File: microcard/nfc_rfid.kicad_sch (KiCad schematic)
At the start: 39 parts, among them Q7 2N7002, U6 ST25R3916-AQWT, X1 XRCGB27M120F3M00R0

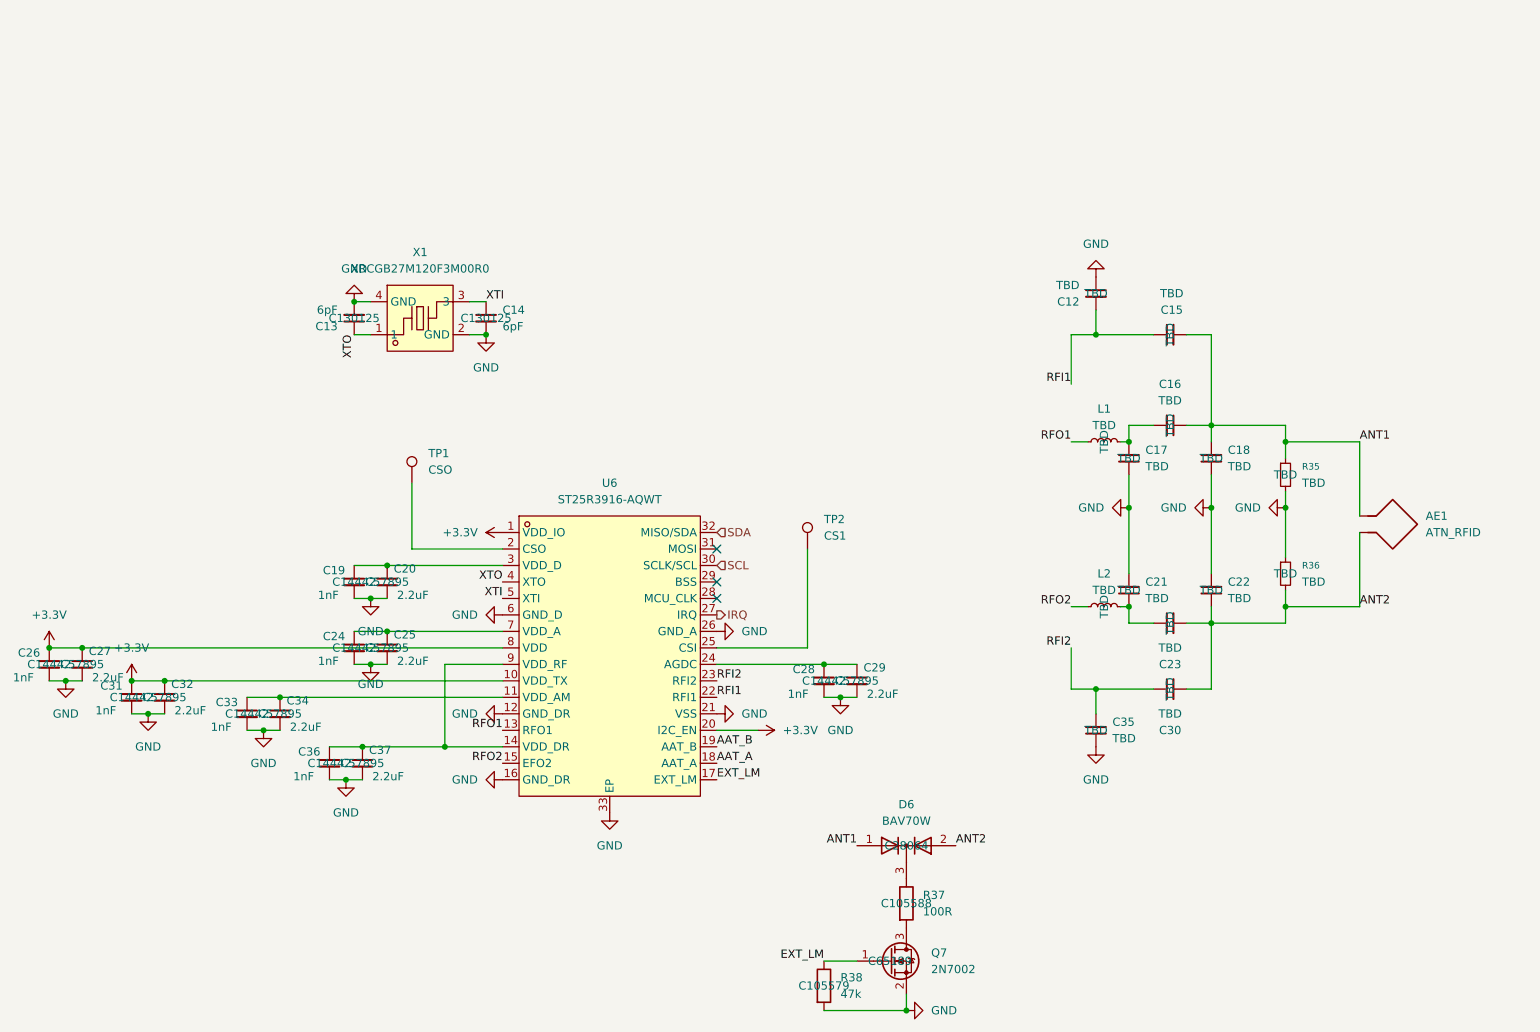
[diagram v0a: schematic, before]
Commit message: wide render
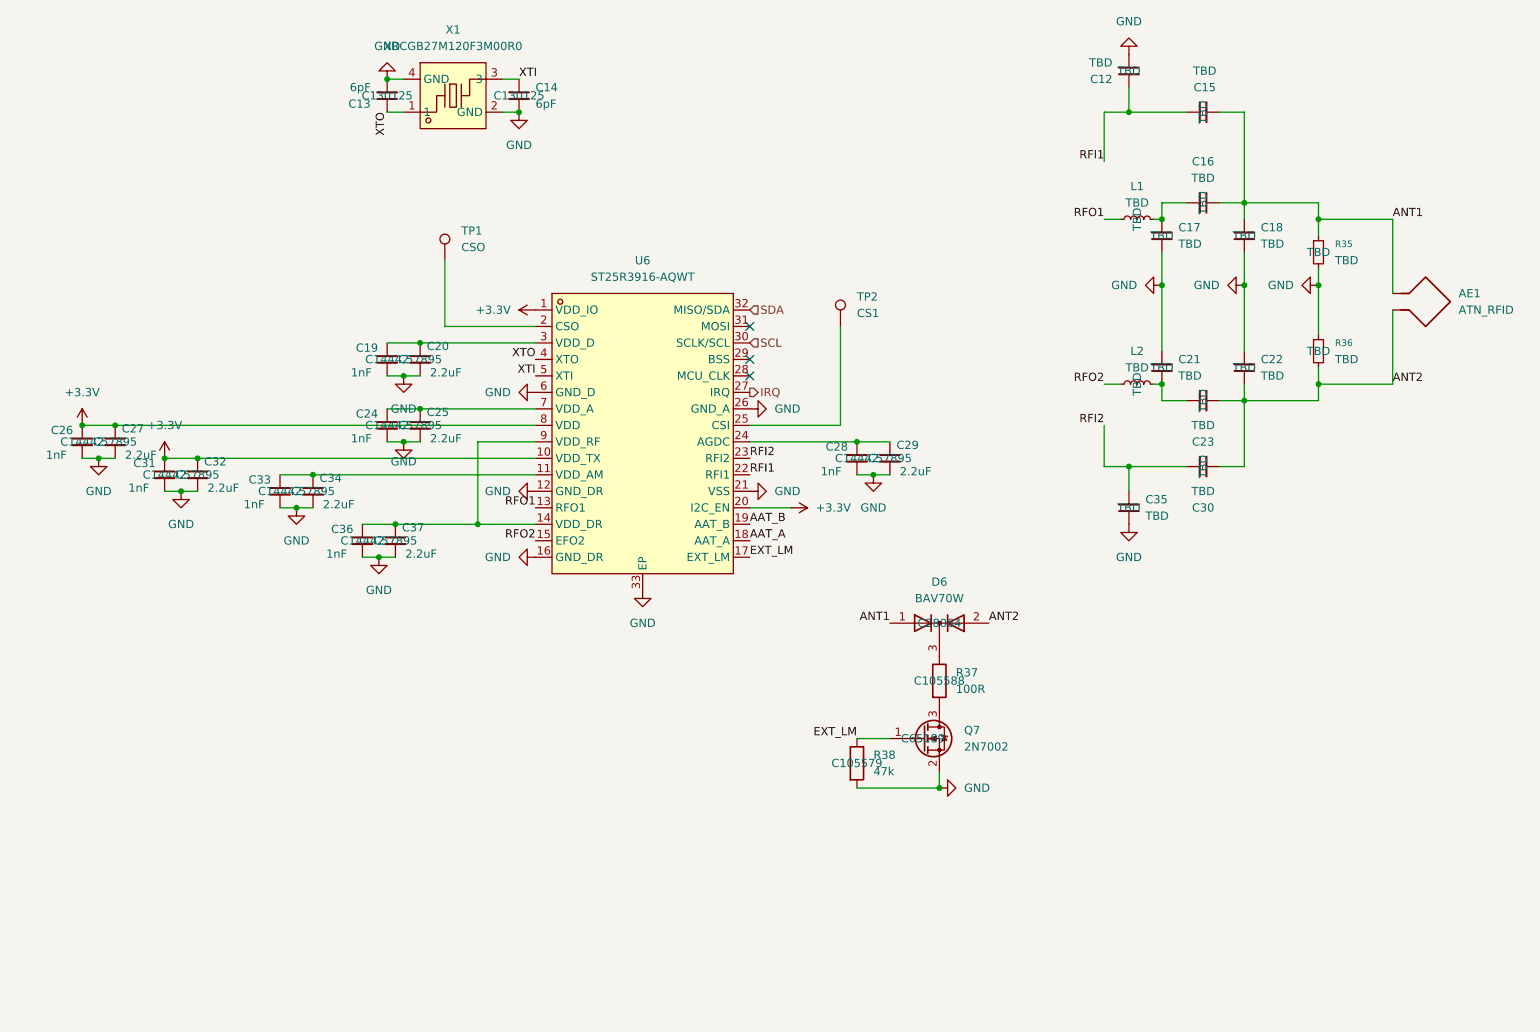
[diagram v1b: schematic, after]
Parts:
- C12, C15, C16, C17, C18, C21, C22, C23, C30, C35: footprint Capacitor_SMD:C_0603_1608Metric_Pad1.08x0.95mm_HandSolder -> Capacitor_SMD:C_0402_1005Metric
- C13, C14, C20, C25, C27, C29, C32, C34, C37: footprint Capacitor_SMD:C_0603_1608Metric_Pad1.08x0.95mm_HandSolder -> Capacitor_SMD:C_0603_1608Metric
- C19, C24, C26, C28, C31, C33, C36: footprint Capacitor_SMD:C_0402_1005Metric_Pad0.74x0.62mm_HandSolder -> Capacitor_SMD:C_0402_1005Metric
- L1, L2: footprint Inductor_SMD:L_0603_1608Metric_Pad1.05x0.95mm_HandSolder -> Inductor_SMD:L_0402_1005Metric
- R35, R36, R37, R38: footprint Resistor_SMD:R_0603_1608Metric_Pad0.98x0.95mm_HandSolder -> Resistor_SMD:R_0603_1608Metric
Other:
- moved on the sheet: AE1, C12, C13, C14, C15, C16, C17, C18, C19, C20, C21, C22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
